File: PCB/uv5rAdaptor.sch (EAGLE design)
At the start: 2 parts

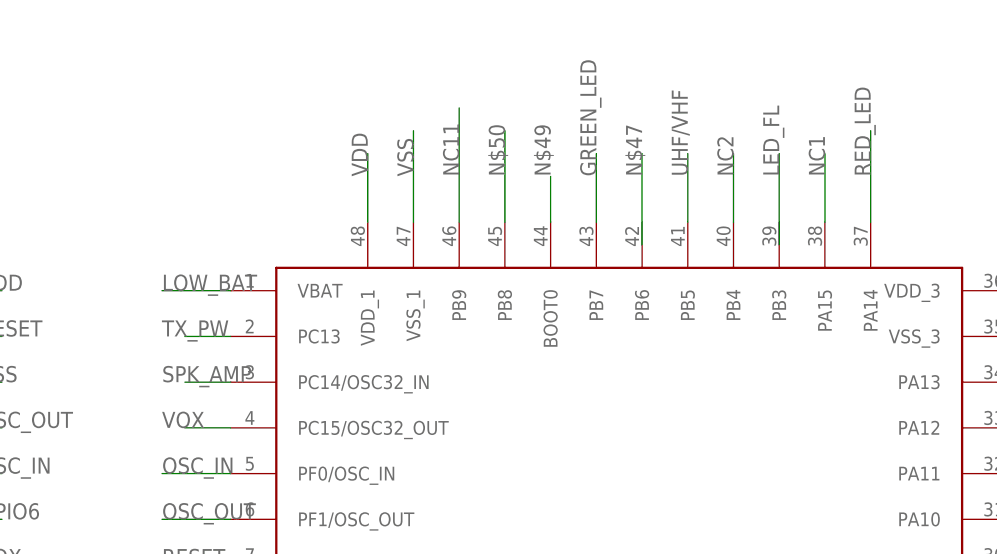
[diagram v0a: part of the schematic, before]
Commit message: More routing
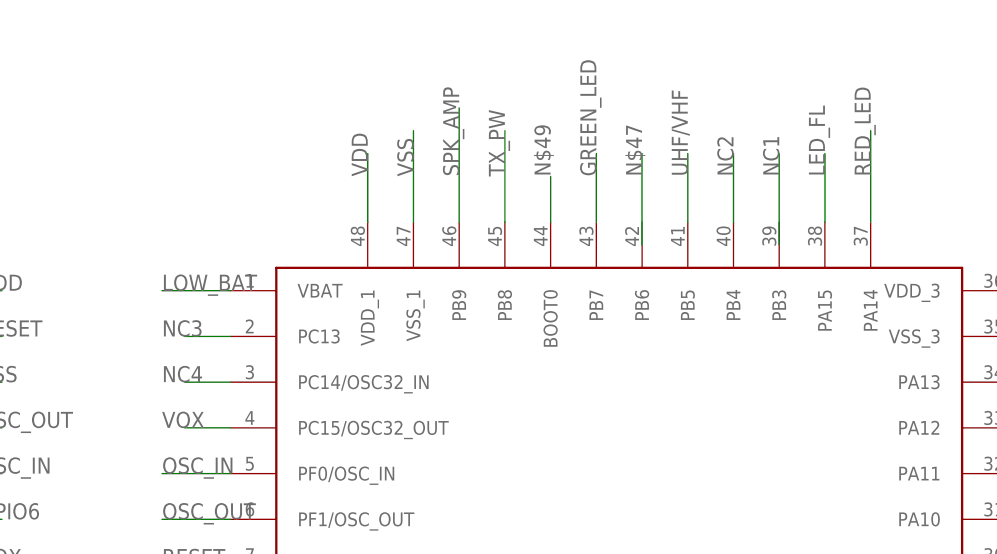
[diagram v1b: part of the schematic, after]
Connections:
- removed net N$50: U$1.PB8
- removed net NC1: U$1.PA15
- removed net NC11: U$1.PB9
- new net NC3: U$1.PC13
- new net NC4: U$1.PC14/OSC32_IN
- net LED_FL: now also U$1.PA15
- net SPK_AMP: now also U$1.PB9; no longer U$1.PC14/OSC32_IN
- net TX_PW: now also U$1.PB8; no longer U$1.PC13

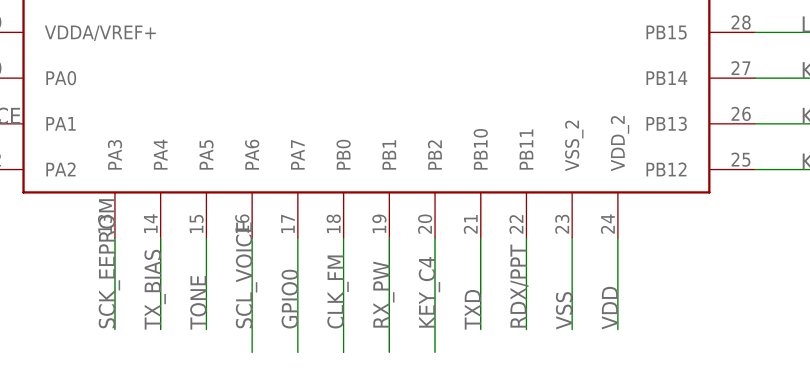
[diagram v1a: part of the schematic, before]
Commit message: More traces
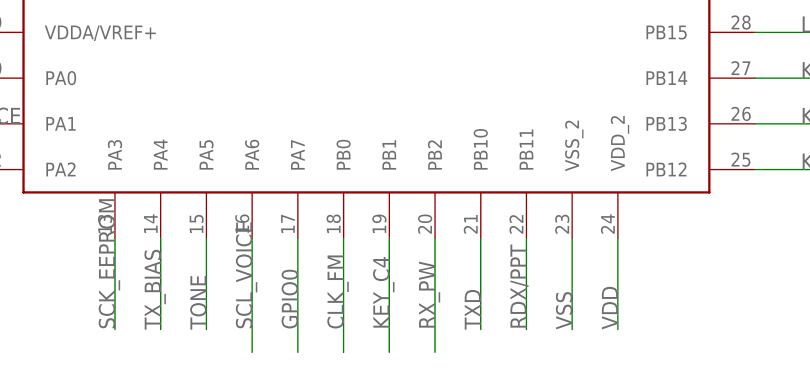
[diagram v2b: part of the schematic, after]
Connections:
- net KEY_C4: now also U$1.PB1; no longer U$1.PB2
- net RX_PW: now also U$1.PB2; no longer U$1.PB1
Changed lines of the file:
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@@
 </segment>
 <segment>
-<pinref part="U$1" gate="G$1" pin="PB2"/>
-<wire x1="142.24" y1="2.54" x2="142.24" y2="-10.16" width="0.1524" layer="91"/>
-<label x="142.24" y="-7.62" size="1.778" layer="95" rot="R90"/>
+<pinref part="U$1" gate="G$1" pin="PB1"/>
+<wire x1="137.16" y1="2.54" x2="137.16" y2="-10.16" width="0.1524" layer="91"/>
+<label x="137.16" y="-7.62" size="1.778" layer="95" rot="R90"/>
 </segment>
 </net>
@@
 </segment>
 <segment>
-<pinref part="U$1" gate="G$1" pin="PB1"/>
-<wire x1="137.16" y1="2.54" x2="137.16" y2="-10.16" width="0.1524" layer="91"/>
-<label x="137.16" y="-7.62" size="1.778" layer="95" rot="R90"/>
+<pinref part="U$1" gate="G$1" pin="PB2"/>
+<wire x1="142.24" y1="2.54" x2="142.24" y2="-10.16" width="0.1524" layer="91"/>
+<label x="142.24" y="-7.62" size="1.778" layer="95" rot="R90"/>
 </segment>
 </net>
